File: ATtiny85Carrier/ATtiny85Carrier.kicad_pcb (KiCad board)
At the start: 2 copper layers, 17 parts, among them J2 Header, J3 GND Header, SW1 Power_SW, U1 ATtiny85-20PU, U2 L78L05_TO92

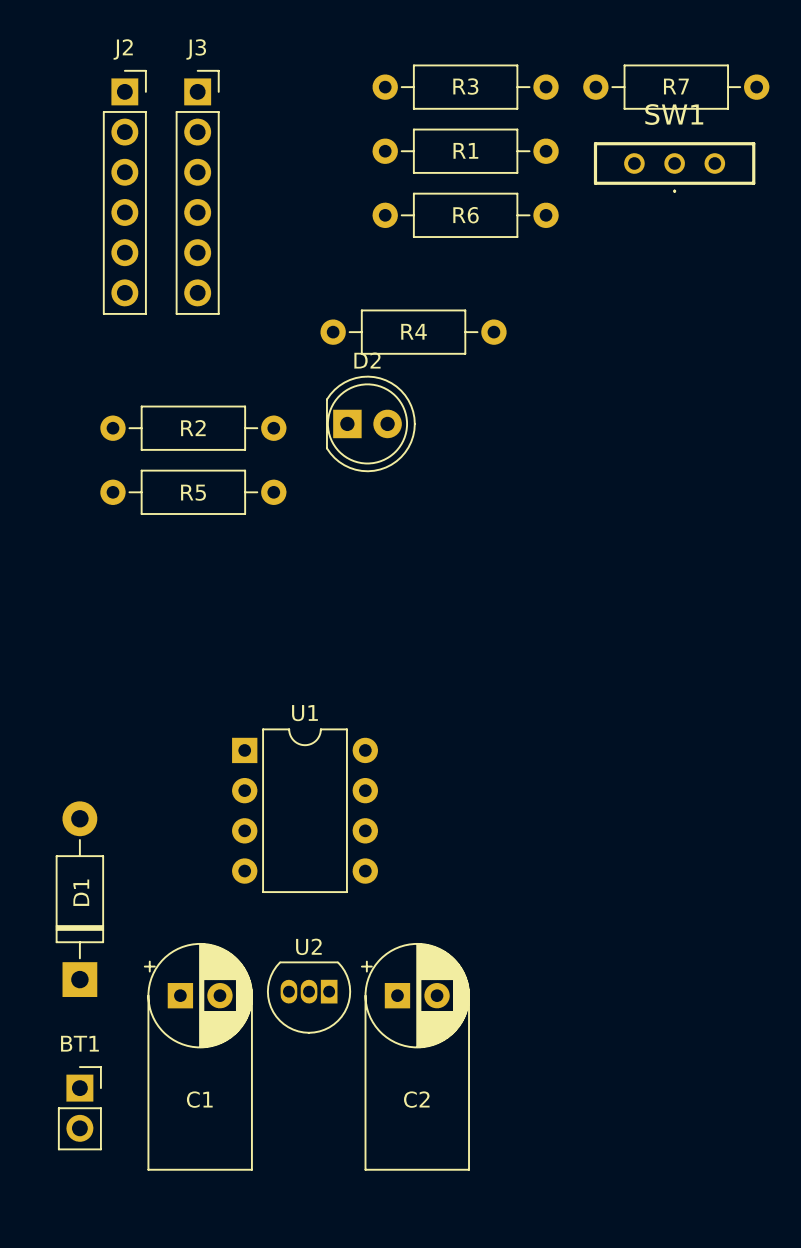
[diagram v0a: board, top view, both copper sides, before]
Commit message: Finalized and exported board
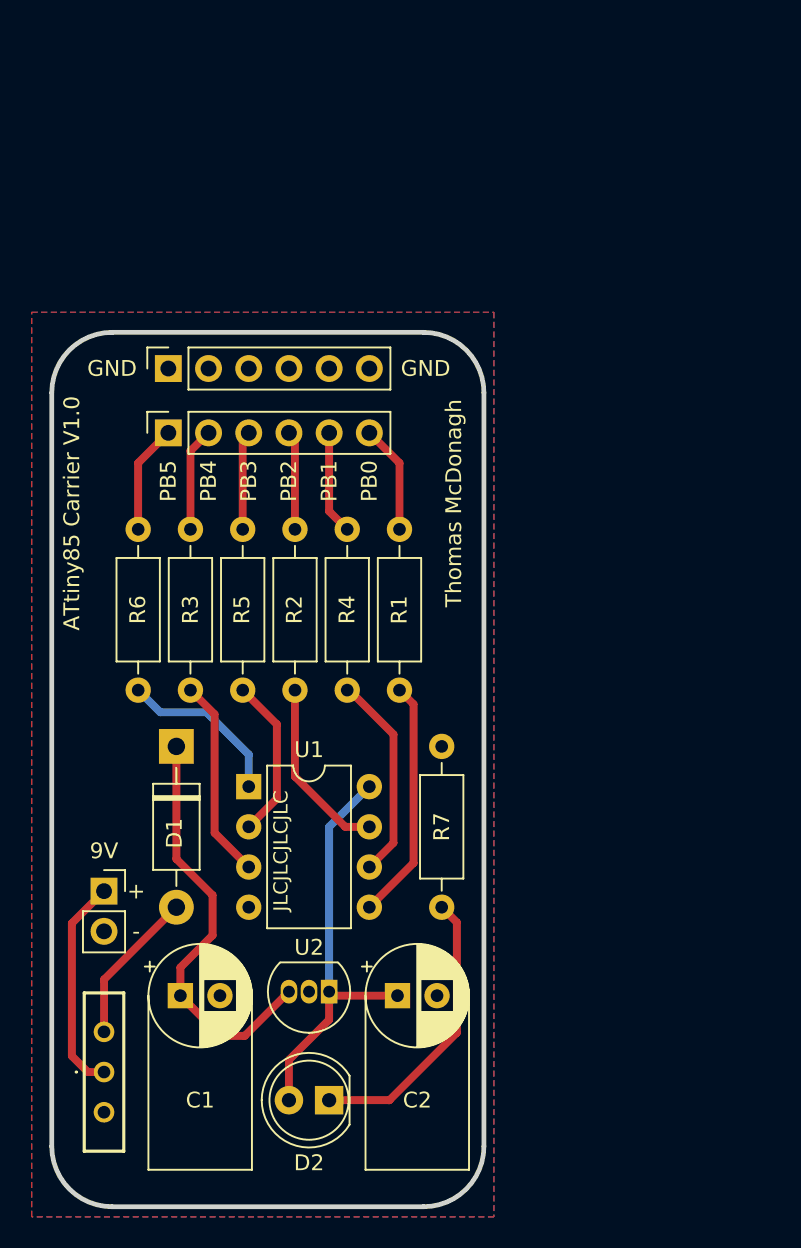
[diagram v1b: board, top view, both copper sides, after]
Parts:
- added G***: LOGO, libraries:attiny85Image, B.Cu at (127.0, 125.7)
- moved SW1 67.8 mm to (116.3, 147.1), turned to 270 degrees
- moved R7 42.8 mm to (137.7, 126.5), turned to 270 degrees
- moved D2 42.7 mm to (130.6, 148.8), turned to 180 degrees
- moved R3 30.5 mm to (121.8, 112.8), turned to 270 degrees
- moved R6 25.2 mm to (118.5, 112.8), turned to 270 degrees
- moved R1 23.9 mm to (135.0, 112.8), turned to 270 degrees
- moved J2 21.7 mm to (120.4, 106.7), turned to 90 degrees
- moved J3 17.6 mm to (120.4, 102.6), turned to 90 degrees
- moved D1 15.9 mm to (120.9, 126.5), turned to 270 degrees
- moved R2 13.2 mm to (128.4, 112.8), turned to 270 degrees
- moved BT1 12.5 mm to (116.3, 135.6)
- moved R4 12.5 mm to (131.7, 112.8), turned to 270 degrees
- moved R5 8.52 mm to (125.1, 112.8), turned to 270 degrees
- moved U1 2.30 mm to (125.5, 129.0)
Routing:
- net Net-(C1-Pad1): track 0.00 -> 26.6 mm
- net +5V: track 0.00 -> 26.3 mm
- net Net-(D2-Pad1): track 0.00 -> 18.2 mm
- net Net-(R1-Pad2): track 0.00 -> 15.2 mm
- net Net-(BT1-Pad1): track 0.00 -> 13.7 mm
- net Net-(R4-Pad2): track 0.00 -> 13.1 mm
- net Net-(R3-Pad2): track 0.00 -> 12.7 mm
- net Net-(R2-Pad2): track 0.00 -> 11.5 mm
- net Net-(R6-Pad2): track 0.00 -> 10.7 mm
- net Net-(R5-Pad2): track 0.00 -> 10.3 mm
- net +9V: track 0.00 -> 9.77 mm
- net Net-(J2-Pad6): track 0.00 -> 6.89 mm
- net Net-(J2-Pad1): track 0.00 -> 6.89 mm
- net Net-(J2-Pad2): track 0.00 -> 6.57 mm
- net Net-(J2-Pad5): track 0.00 -> 6.57 mm
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- added copper zone on B.Cu, net GND
- added copper zone on F.Cu, net GND
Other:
- board outline added: 27.3 x 55.2 mm
- board text added: "+"
- board text added: "-"
- board text added: "9V"
- board text added: "ATtiny85 Carrier V1.0"
- board text added: "GND"
- board text added: "JLCJLCJLCJLC"
- board text added: "PB0"
- board text added: "PB1"
- board text added: "PB2"
- board text added: "PB3"
- board text added: "PB4"
- board text added: "PB5"
- board text added: "Thomas McDonagh"
